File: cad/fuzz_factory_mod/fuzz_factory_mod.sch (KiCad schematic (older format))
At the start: 2 parts

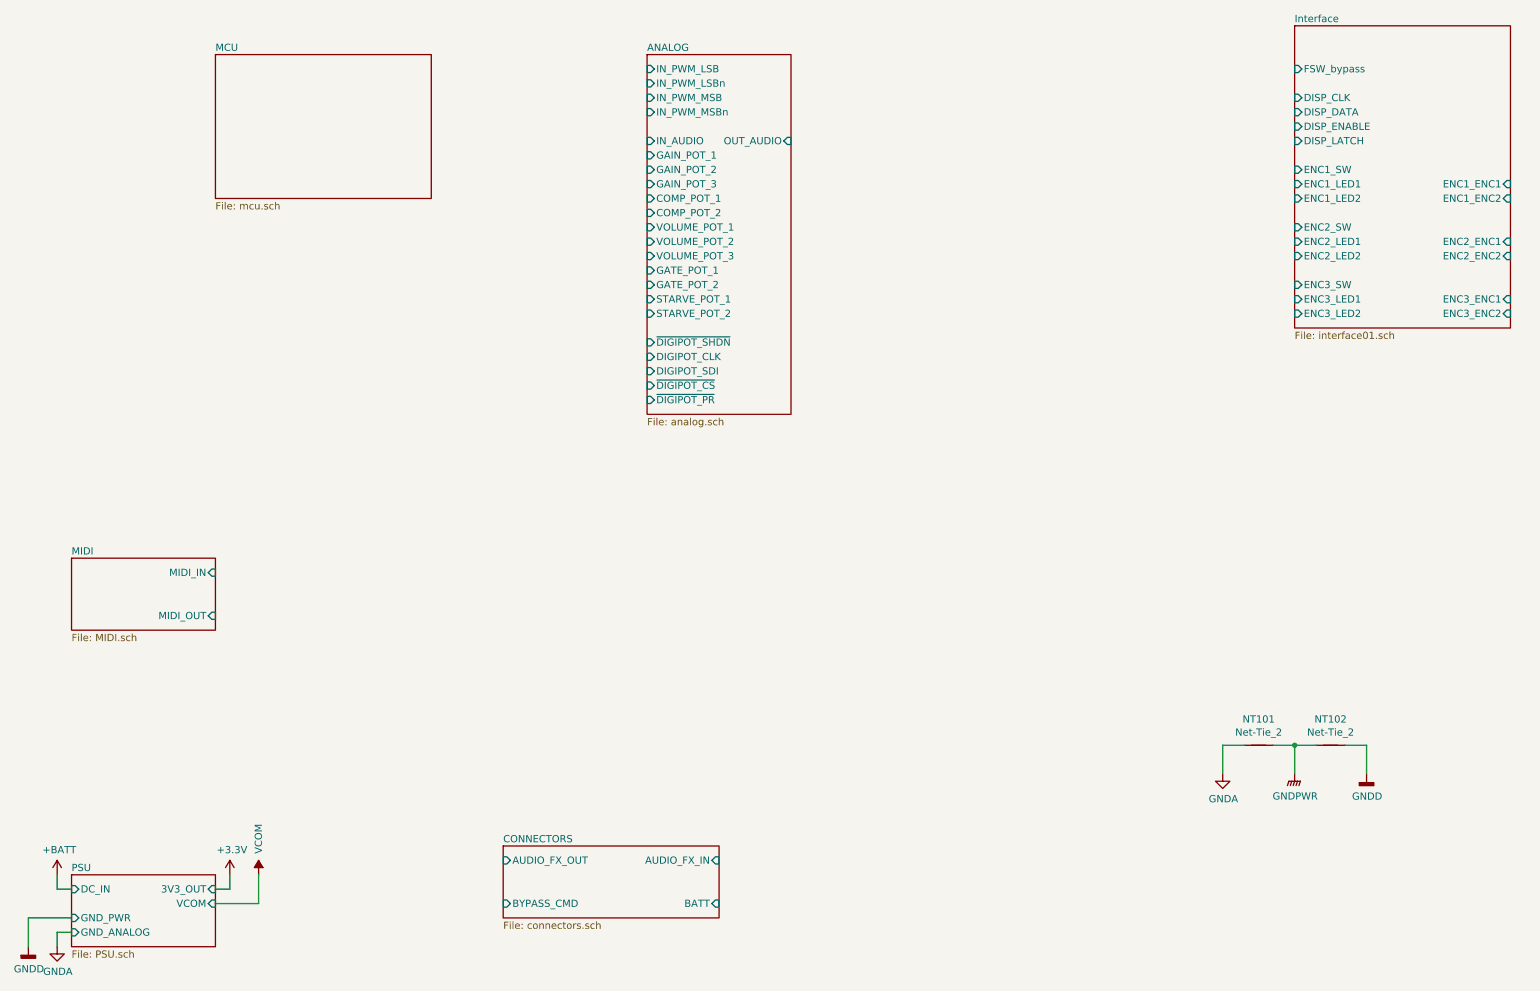
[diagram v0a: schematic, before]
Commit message: Continued schematic.
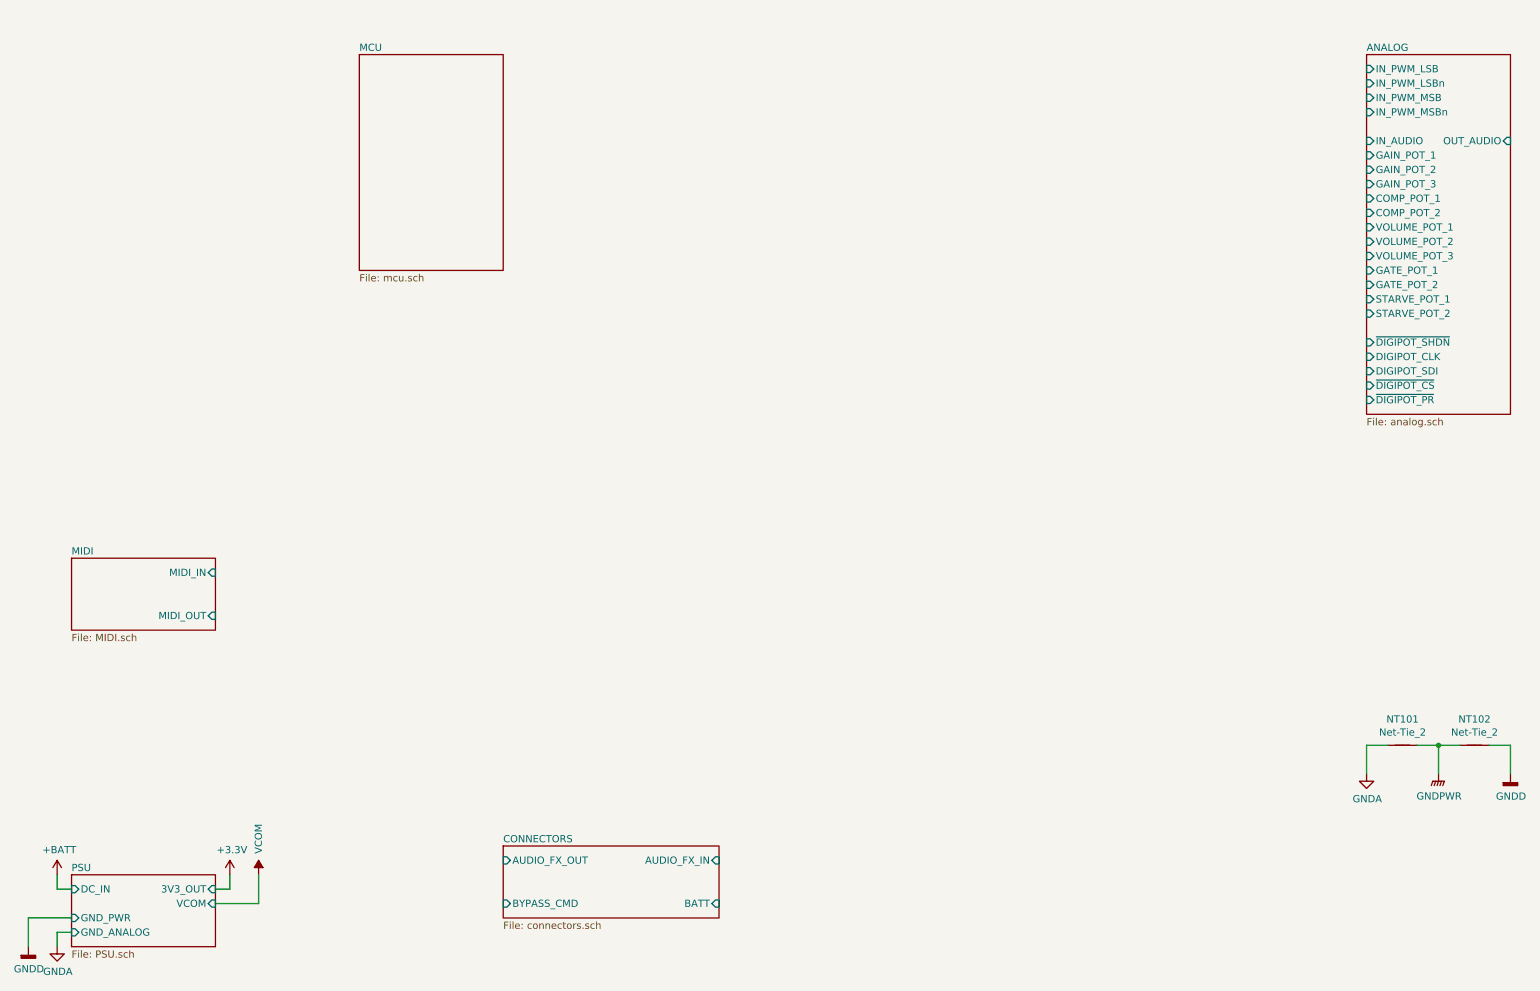
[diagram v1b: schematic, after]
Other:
- moved on the sheet: NT101, NT102
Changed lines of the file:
@@
 $Descr A4 11693 8268
 encoding utf-8
-Sheet 1 22
+Sheet 1 26
 Title ""
 Date ""
@@
 $EndDescr
 $Sheet
-S 2000 1000 1500 1000
+S 3000 1000 1000 1500
 U 5DE4AD26
 F0 "MCU" 50
@@
 $EndSheet
 $Sheet
-S 5000 1000 1000 2500
+S 10000 1000 1000 2500
 U 5DE4AD88
 F0 "ANALOG" 50
 F1 "analog.sch" 50
-F2 "GAIN_POT_1" I L 5000 1700 50
-F3 "GAIN_POT_2" I L 5000 1800 50
-F4 "GAIN_POT_3" I L 5000 1900 50
-F5 "COMP_POT_1" I L 5000 2000 50
-F6 "COMP_POT_2" I L 5000 2100 50
-F7 "VOLUME_POT_1" I L 5000 2200 50
-F8 "VOLUME_POT_2" I L 5000 2300 50
-F9 "VOLUME_POT_3" I L 5000 2400 50
-F10 "GATE_POT_1" I L 5000 2500 50
-F11 "GATE_POT_2" I L 5000 2600 50
-F12 "IN_AUDIO" I L 5000 1600 50
-F13 "IN_PWM_LSB" I L 5000 1100 50
-F14 "IN_PWM_LSBn" I L 5000 1200 50
-F15 "IN_PWM_MSB" I L 5000 1300 50
-F16 "IN_PWM_MSBn" I L 5000 1400 50
-F17 "STARVE_POT_1" I L 5000 2700 50
-F18 "STARVE_POT_2" I L 5000 2800 50
-F19 "OUT_AUDIO" I R 6000 1600 50
-F20 "~DIGIPOT_SHDN" I L 5000 3000 50
-F21 "DIGIPOT_CLK" I L 5000 3100 50
-F22 "DIGIPOT_SDI" I L 5000 3200 50
-F23 "~DIGIPOT_CS" I L 5000 3300 50
-F24 "~DIGIPOT_PR" I L 5000 3400 50
+F2 "GAIN_POT_1" I L 10000 1700 50
+F3 "GAIN_POT_2" I L 10000 1800 50
+F4 "GAIN_POT_3" I L 10000 1900 50
+F5 "COMP_POT_1" I L 10000 2000 50
+F6 "COMP_POT_2" I L 10000 2100 50
+F7 "VOLUME_POT_1" I L 10000 2200 50
+F8 "VOLUME_POT_2" I L 10000 2300 50
+F9 "VOLUME_POT_3" I L 10000 2400 50
+F10 "GATE_POT_1" I L 10000 2500 50
+F11 "GATE_POT_2" I L 10000 2600 50
+F12 "IN_AUDIO" I L 10000 1600 50
+F13 "IN_PWM_LSB" I L 10000 1100 50
+F14 "IN_PWM_LSBn" I L 10000 1200 50
+F15 "IN_PWM_MSB" I L 10000 1300 50
+F16 "IN_PWM_MSBn" I L 10000 1400 50
+F17 "STARVE_POT_1" I L 10000 2700 50
+F18 "STARVE_POT_2" I L 10000 2800 50
+F19 "OUT_AUDIO" I R 11000 1600 50
+F20 "~DIGIPOT_SHDN" I L 10000 3000 50
+F21 "DIGIPOT_CLK" I L 10000 3100 50
+F22 "DIGIPOT_SDI" I L 10000 3200 50
+F23 "~DIGIPOT_CS" I L 10000 3300 50
+F24 "~DIGIPOT_PR" I L 10000 3400 50
 $EndSheet
 $Sheet
@@
 L power:GNDA #PWR0106
 U 1 1 5E05A512
-P 9000 6000
-F 0 "#PWR0106" H 9000 5750 50  0001 C CNN
-F 1 "GNDA" H 9005 5827 50  0000 C CNN
-F 2 "" H 9000 6000 50  0001 C CNN
-F 3 "" H 9000 6000 50  0001 C CNN
-	1    9000 6000
-	1    0    0    -1
-$EndComp
-$Comp
-L power:GNDPWR #PWR0107
-U 1 1 5E05AF8B
-P 9500 6000
-F 0 "#PWR0107" H 9500 5800 50  0001 C CNN
-F 1 "GNDPWR" H 9504 5846 50  0000 C CNN
-F 2 "" H 9500 5950 50  0001 C CNN
-F 3 "" H 9500 5950 50  0001 C CNN
-	1    9500 6000
-	1    0    0    -1
-$EndComp
-$Comp
-L power:GNDD #PWR0108
-U 1 1 5E05B768
 P 10000 6000
-F 0 "#PWR0108" H 10000 5750 50  0001 C CNN
-F 1 "GNDD" H 10004 5845 50  0000 C CNN
+F 0 "#PWR0106" H 10000 5750 50  0001 C CNN
+F 1 "GNDA" H 10005 5827 50  0000 C CNN
 F 2 "" H 10000 6000 50  0001 C CNN
 F 3 "" H 10000 6000 50  0001 C CNN
@@
 $EndComp
 $Comp
+L power:GNDPWR #PWR0107
+U 1 1 5E05AF8B
+P 10500 6000
+F 0 "#PWR0107" H 10500 5800 50  0001 C CNN
+F 1 "GNDPWR" H 10504 5846 50  0000 C CNN
+F 2 "" H 10500 5950 50  0001 C CNN
+F 3 "" H 10500 5950 50  0001 C CNN
+	1    10500 6000
+	1    0    0    -1
+$EndComp
+$Comp
+L power:GNDD #PWR0108
+U 1 1 5E05B768
+P 11000 6000
+F 0 "#PWR0108" H 11000 5750 50  0001 C CNN
+F 1 "GNDD" H 11004 5845 50  0000 C CNN
+F 2 "" H 11000 6000 50  0001 C CNN
+F 3 "" H 11000 6000 50  0001 C CNN
+	1    11000 6000
+	1    0    0    -1
+$EndComp
+$Comp
 L Device:Net-Tie_2 NT101
 U 1 1 5E05BC9C
-P 9250 5800
-F 0 "NT101" H 9250 5981 50  0000 C CNN
-F 1 "Net-Tie_2" H 9250 5890 50  0000 C CNN
-F 2 "Oddities:NetTie-II" H 9250 5800 50  0001 C CNN
-F 3 "~" H 9250 5800 50  0001 C CNN
-	1    9250 5800
+P 10250 5800
+F 0 "NT101" H 10250 5981 50  0000 C CNN
+F 1 "Net-Tie_2" H 10250 5890 50  0000 C CNN
+F 2 "Oddities:NetTie-II" H 10250 5800 50  0001 C CNN
+F 3 "~" H 10250 5800 50  0001 C CNN
+	1    10250 5800
 	1    0    0    -1
 $EndComp
@@
 L Device:Net-Tie_2 NT102
 U 1 1 5E05C2E4
-P 9750 5800
-F 0 "NT102" H 9750 5981 50  0000 C CNN
-F 1 "Net-Tie_2" H 9750 5890 50  0000 C CNN
-F 2 "Oddities:NetTie-II" H 9750 5800 50  0001 C CNN
-F 3 "~" H 9750 5800 50  0001 C CNN
-	1    9750 5800
+P 10750 5800
+F 0 "NT102" H 10750 5981 50  0000 C CNN
+F 1 "Net-Tie_2" H 10750 5890 50  0000 C CNN
+F 2 "Oddities:NetTie-II" H 10750 5800 50  0001 C CNN
+F 3 "~" H 10750 5800 50  0001 C CNN
+	1    10750 5800
 	1    0    0    -1
 $EndComp
 Wire Wire Line
+	11000 6000 11000 5800
+Wire Wire Line
+	11000 5800 10850 5800
+Wire Wire Line
+	10650 5800 10500 5800
+Wire Wire Line
+	10500 6000 10500 5800
+Connection ~ 10500 5800
+Wire Wire Line
+	10500 5800 10350 5800
+Wire Wire Line
 	10000 6000 10000 5800
 Wire Wire Line
-	10000 5800 9850 5800
-Wire Wire Line
-	9650 5800 9500 5800
-Wire Wire Line
-	9500 6000 9500 5800
-Connection ~ 9500 5800
-Wire Wire Line
-	9500 5800 9350 5800
-Wire Wire Line
-	9000 6000 9000 5800
-Wire Wire Line
-	9000 5800 9150 5800
-$Sheet
-S 9500 800  1500 2100
-U 5E083283
-F0 "Interface" 50
-F1 "interface01.sch" 50
-F2 "DISP_CLK" I L 9500 1300 50
-F3 "DISP_DATA" I L 9500 1400 50
-F4 "DISP_ENABLE" I L 9500 1500 50
-F5 "DISP_LATCH" I L 9500 1600 50
-F6 "ENC1_SW" I L 9500 1800 50
-F7 "ENC1_LED1" I L 9500 1900 50
-F8 "ENC1_LED2" I L 9500 2000 50
-F9 "ENC1_ENC1" I R 11000 1900 50
-F10 "ENC1_ENC2" I R 11000 2000 50
-F11 "FSW_bypass" I L 9500 1100 50
-F12 "ENC2_SW" I L 9500 2200 50
-F13 "ENC2_LED1" I L 9500 2300 50
-F14 "ENC2_LED2" I L 9500 2400 50
-F15 "ENC2_ENC1" I R 11000 2300 50
-F16 "ENC2_ENC2" I R 11000 2400 50
-F17 "ENC3_SW" I L 9500 2600 50
-F18 "ENC3_LED1" I L 9500 2700 50
-F19 "ENC3_LED2" I L 9500 2800 50
-F20 "ENC3_ENC1" I R 11000 2700 50
-F21 "ENC3_ENC2" I R 11000 2800 50
-$EndSheet
+	10000 5800 10150 5800
 $Sheet
 S 1000 6700 1000 500
